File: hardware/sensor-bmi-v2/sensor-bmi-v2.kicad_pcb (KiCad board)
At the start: 2 copper layers, 10 x 40 mm, 27 parts, among them J1 JST SH1.0, Q1 BSS138, Q2 BSS138, U1 LN1134A182MR-G, U2 MAX30102, U3 LIS2MDL, U4 BMI160

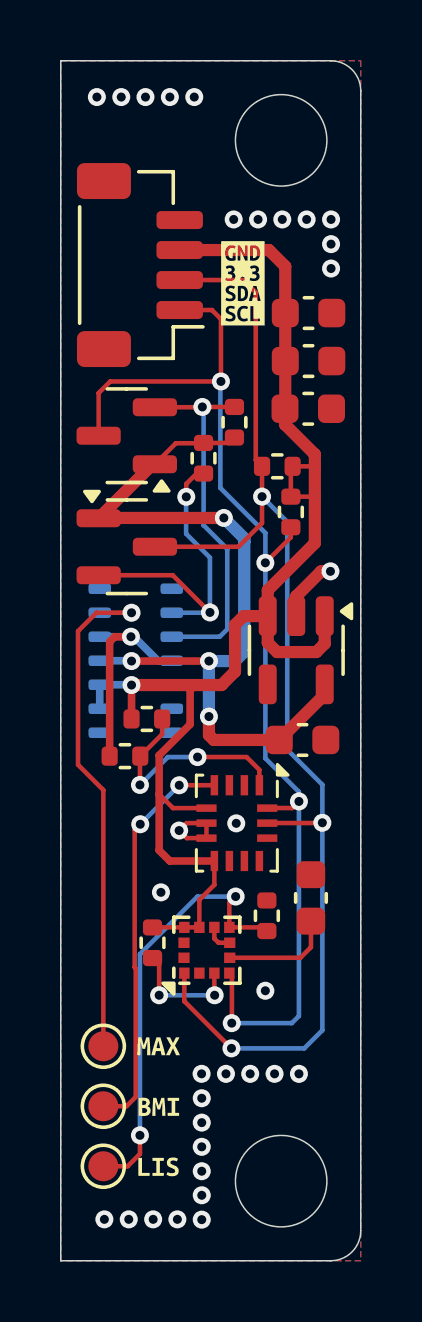
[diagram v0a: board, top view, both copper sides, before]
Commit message: Update for poduction
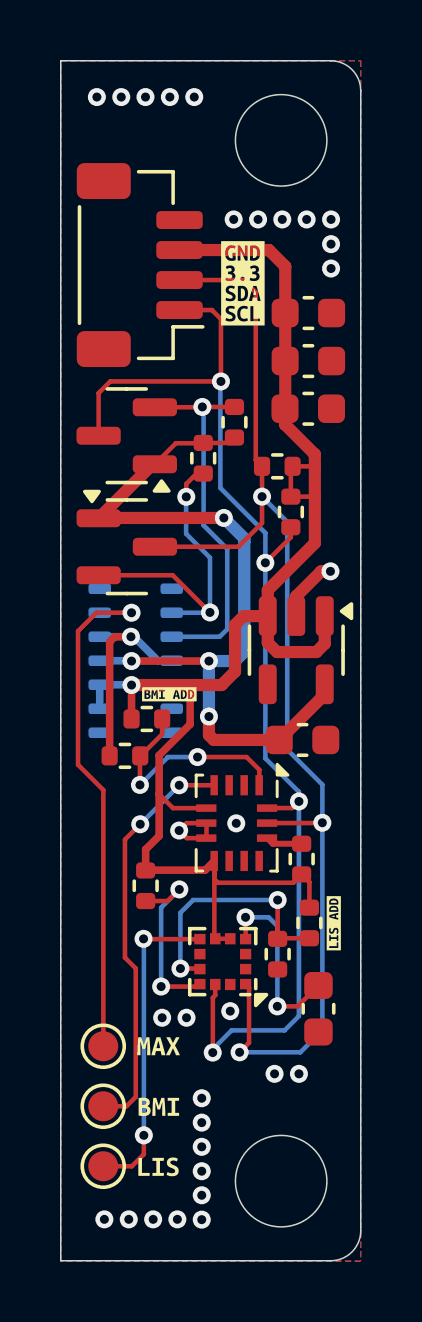
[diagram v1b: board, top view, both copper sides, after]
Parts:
- removed C1: 1uF 16V, Capacitor_SMD:C_0603_1608Metric
- removed C2: 2.2uF 16V, Capacitor_SMD:C_0603_1608Metric
- removed C3, C4, C5: 100nF 16V, Capacitor_SMD:C_0603_1608Metric
- removed J1: JST SH1.0, Connector_JST:JST_SH_BM04B-SRSS-TB_1x04-1MP_P1.00mm_Vertical
- removed Q1, Q2: BSS138, Package_TO_SOT_SMD:SOT-23
- removed R1, R2, R3, R4, R5, R6, R8: 10K, Resistor_SMD:R_0402_1005Metric
- removed R7: 0R, Resistor_SMD:R_0402_1005Metric
- removed TP1: MAX_INT, TestPoint:TestPoint_Pad_D1.0mm
- removed TP2: LIS_INT, TestPoint:TestPoint_Pad_D1.0mm
- removed TP3: BMI_INT, TestPoint:TestPoint_Pad_D1.0mm
- removed U1: LN1134A182MR-G, Package_TO_SOT_SMD:SOT-23-5
- removed U2: MAX30102, OptoDevice:Maxim_OLGA-14_3.3x5.6mm_P0.8mm
- removed U3: LIS2MDL, Package_LGA:LGA-12_2x2mm_P0.5mm
- removed U4: BMI160, Package_LGA:Bosch_LGA-14_3x2.5mm_P0.5mm
- added C41: 1uF 16V, Capacitor_SMD:C_0603_1608Metric, F.Cu at (140.8, 112.2)
- added C42: 2.2uF 16V, Capacitor_SMD:C_0603_1608Metric, F.Cu at (140.6, 124.8)
- added C43: 100nF 10V, Capacitor_SMD:C_0603_1608Metric, F.Cu at (141.2, 133.8)
- added C44: 100nF 10V, Capacitor_SMD:C_0603_1608Metric, F.Cu at (140.8, 113.8)
- added C45: 100nF 10V, Capacitor_SMD:C_0603_1608Metric, F.Cu at (140.8, 110.6)
- added J41: JST SH1.0, Connector_JST:JST_SH_BM04B-SRSS-TB_1x04-1MP_P1.00mm_Vertical, F.Cu at (135.2, 109.0)
- added Q41: BSS138, Package_TO_SOT_SMD:SOT-23, F.Cu at (134.8, 118.3)
- added Q42: BSS138, Package_TO_SOT_SMD:SOT-23, F.Cu at (134.8, 114.7)
- added R41: 10K, Resistor_SMD:R_0402_1005Metric, F.Cu at (138.4, 114.2)
- added R42: 10K, Resistor_SMD:R_0402_1005Metric, F.Cu at (137.3, 115.4)
- added R43: 10K, Resistor_SMD:R_0402_1005Metric, F.Cu at (135.4, 129.7)
- added R44: 10K, Resistor_SMD:R_0402_1005Metric, F.Cu at (140.2, 117.2)
- added R45: 10K, Resistor_SMD:R_0402_1005Metric, F.Cu at (139.8, 115.7)
- added R47: DNP, Resistor_SMD:R_0402_1005Metric, F.Cu at (135.4, 124.1)
- added R48: 10K, Resistor_SMD:R_0402_1005Metric, F.Cu at (134.7, 125.3)
- added R49: 10K, Resistor_SMD:R_0402_1005Metric, F.Cu at (140.6, 128.8)
- added R50: DNP, Resistor_SMD:R_0402_1005Metric, F.Cu at (140.9, 130.9)
- added R51: 10K, Resistor_SMD:R_0402_1005Metric, F.Cu at (139.8, 131.9)
- added TP41: MAX_INT, TestPoint:TestPoint_Pad_D1.0mm, F.Cu at (134.0, 135.0)
- added TP42: LIS_INT, TestPoint:TestPoint_Pad_D1.0mm, F.Cu at (134.0, 139.0)
- added TP43: BMI_INT, TestPoint:TestPoint_Pad_D1.0mm, F.Cu at (134.0, 137.0)
- added U41: LN1134A182MR-G, Package_TO_SOT_SMD:SOT-23-5, F.Cu at (140.4, 121.8)
- added U42: MAX30102, OptoDevice:Maxim_OLGA-14_3.3x5.6mm_P0.8mm, B.Cu at (135.1, 122.2)
- added U44: BMI270, Package_LGA:Bosch_LGA-14_3x2.5mm_P0.5mm, F.Cu at (138.4, 127.6)
- added U45: LIS3MDL, Package_LGA:LGA-12_2x2mm_P0.5mm, F.Cu at (138.0, 132.2)
- added kibuzzard-6818BCEF: G***, kibuzzard-6818BCEF, F.Cu at (141.7, 130.9)
- added kibuzzard-6818BD0F: G***, kibuzzard-6818BD0F, F.Cu at (136.2, 123.3)
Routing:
- net Net-(U42-~{INT}): track 0.00 -> 17.3 mm, vias 0 -> 1
- net Net-(U2-~{INT}): track 17.3 -> 0.00 mm, vias 1 -> 0
- net Net-(U3-DRDY): track 14.5 -> 0.00 mm, vias 2 -> 0
- net Net-(U44-INT1): track 0.00 -> 13.7 mm, vias 0 -> 2
- net Net-(U4-INT1): track 13.4 -> 0.00 mm, vias 2 -> 0
- net Net-(U45-INT): track 0.00 -> 10.6 mm, vias 0 -> 2
- net Net-(U45-SDO/SA1): track 0.00 -> 8.29 mm, vias 0 -> 2
- net Net-(U44-SDO): track 0.00 -> 7.56 mm, vias 0 -> 2
- net Net-(U4-SDO): track 7.56 -> 0.00 mm, vias 2 -> 0
- net Net-(U45-C1): track 0.00 -> 6.25 mm, vias 0 -> 2
- net Net-(U45-~{CS}): track 0.00 -> 6.10 mm, vias 0 -> 2
- net +3V3: track 47.0 -> 52.3 mm
- net Net-(U3-~{CS}): track 3.92 -> 0.00 mm, vias 2 -> 0
- net Net-(U3-C1): track 3.72 -> 0.00 mm
- net SDA: track 38.2 -> 39.9 mm
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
